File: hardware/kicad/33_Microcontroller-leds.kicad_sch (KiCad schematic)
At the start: 11 parts, among them CN2301 S4B-XH-A_LF_SN, U69 74AHCT1G125GW,125-JSM, U70 WS2815F

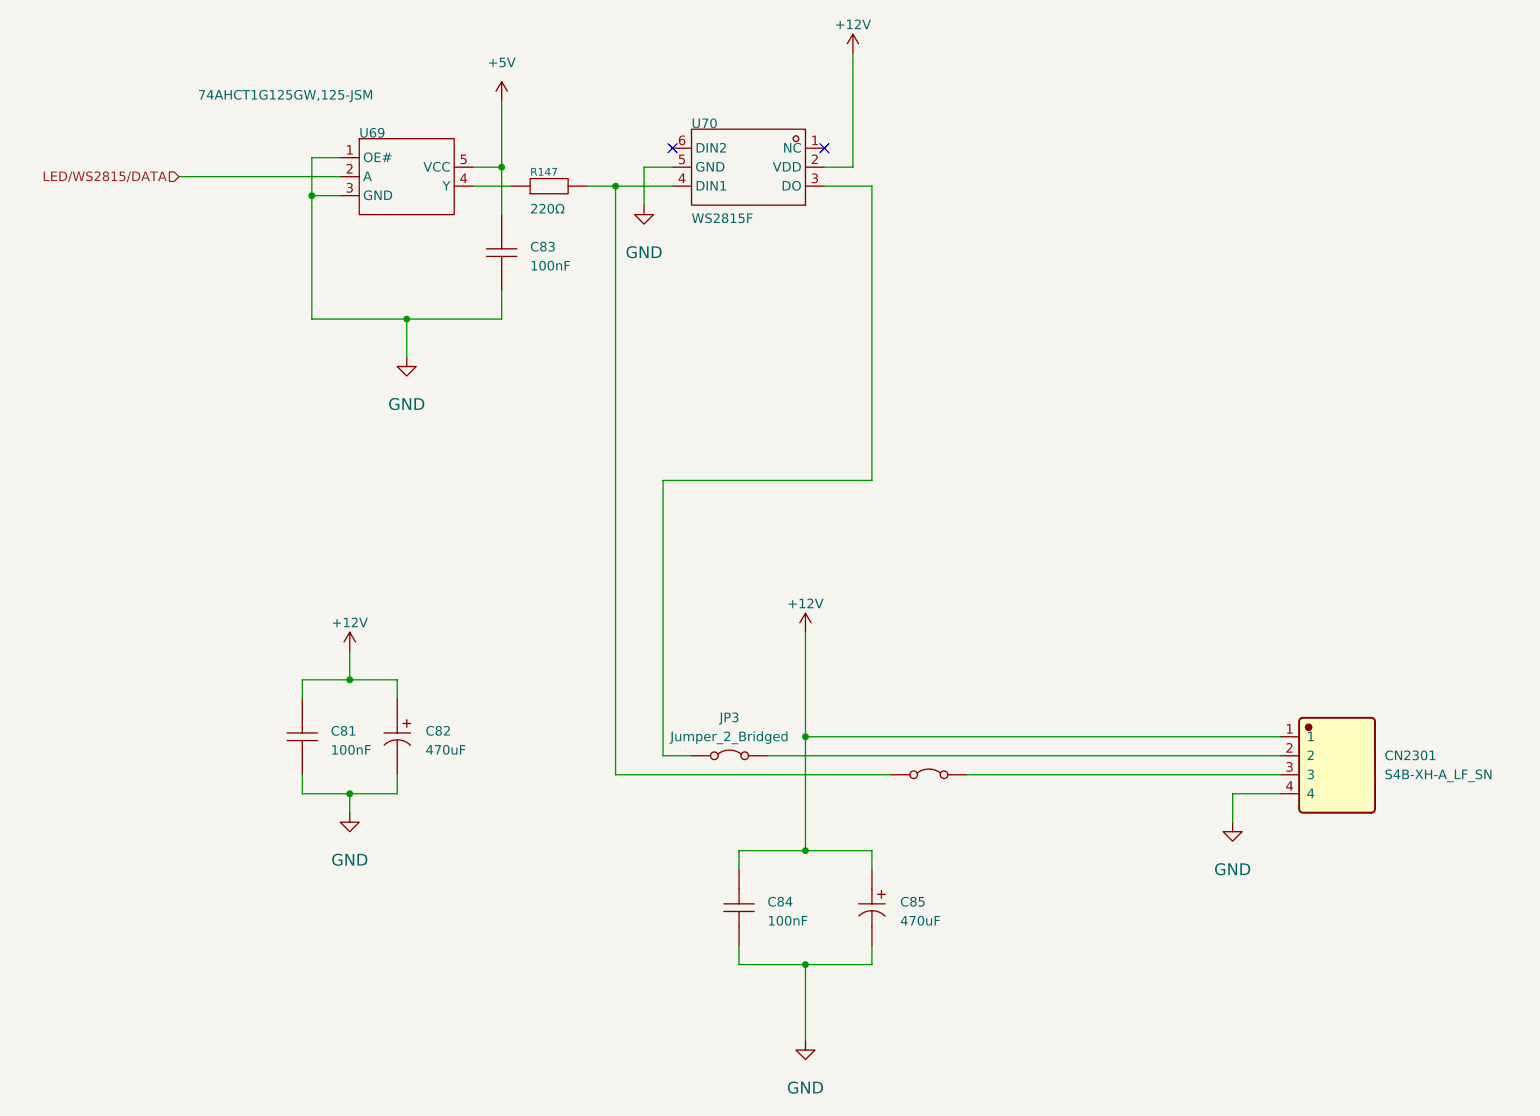
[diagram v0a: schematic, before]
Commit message: leds mostly done
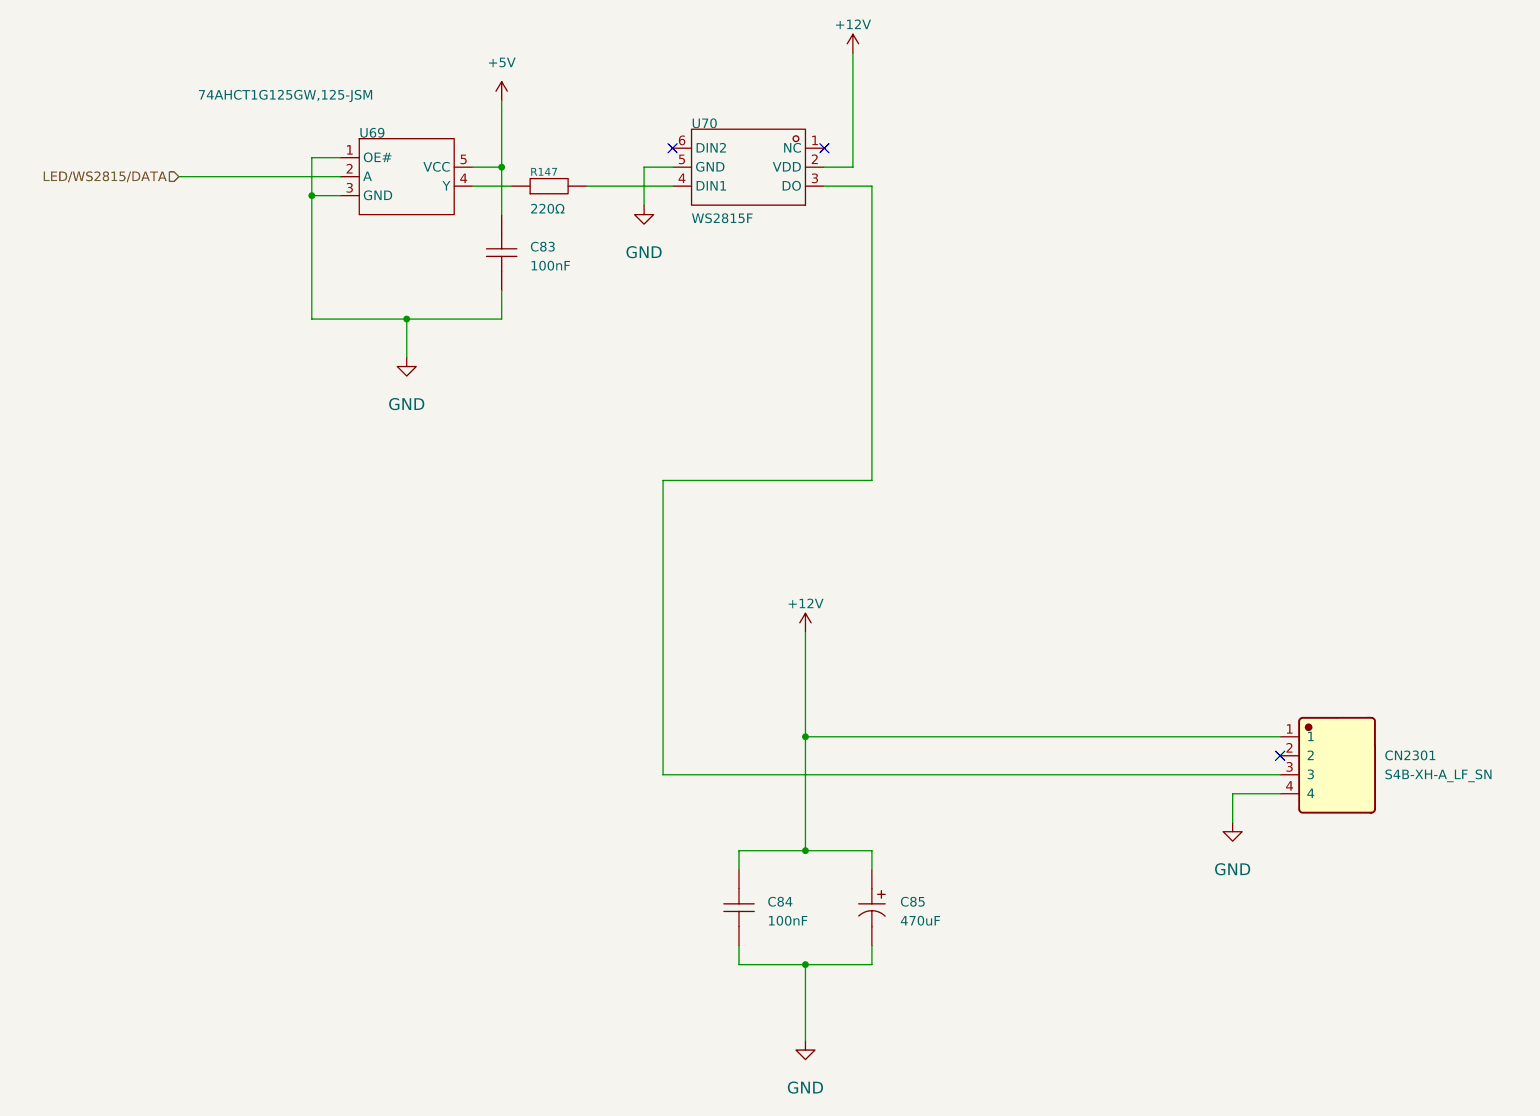
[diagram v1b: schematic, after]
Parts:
- removed C81: 100nF, 5v rail sm-easyedapro:C0603, symbol 5v rail sm-easyedapro:CC0603KRX7R9BB104
- removed C82: 470uF, 5v rail sm-easyedapro:CAP-SMD_BD6.3-L6.6-W6.6-LS7.6-RD, symbol 5v rail sm-easyedapro:RVT1C471M0607
- removed JP2301, JP3: Jumper_2_Bridged, Jumper:SolderJumper-2_P1.3mm_Bridged_RoundedPad1.0x1.5mm, symbol Jumper:Jumper_2_Bridged
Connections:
- net GND: now also C85.2
- net at U70.3 (DO): now also CN2301.3
- no-connect marks 2 -> 3
